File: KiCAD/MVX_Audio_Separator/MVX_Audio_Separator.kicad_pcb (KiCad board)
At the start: 2 copper layers, 30.9 x 26.9 mm, 4 parts, among them J1 3.5mm_vertical, P1 VGA_Female, P2 VGA_Male

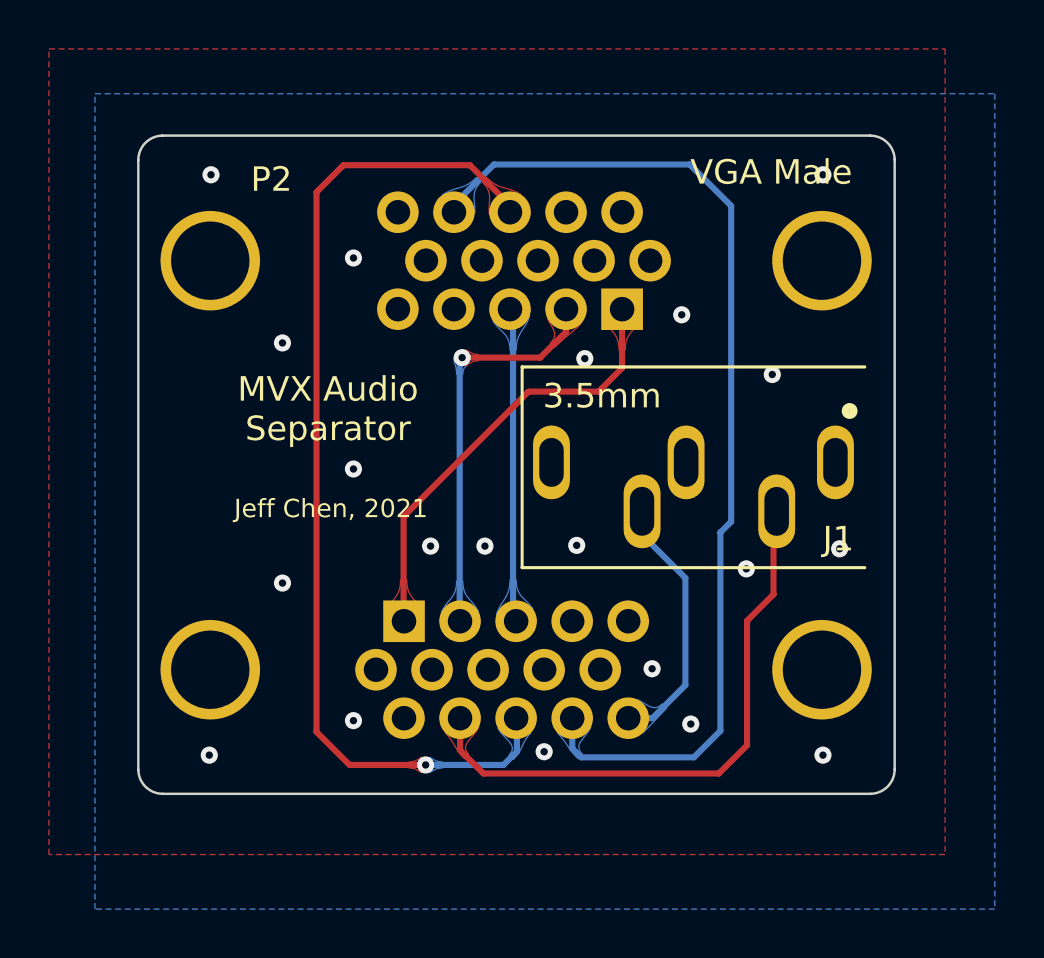
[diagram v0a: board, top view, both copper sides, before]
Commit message: Update PCB
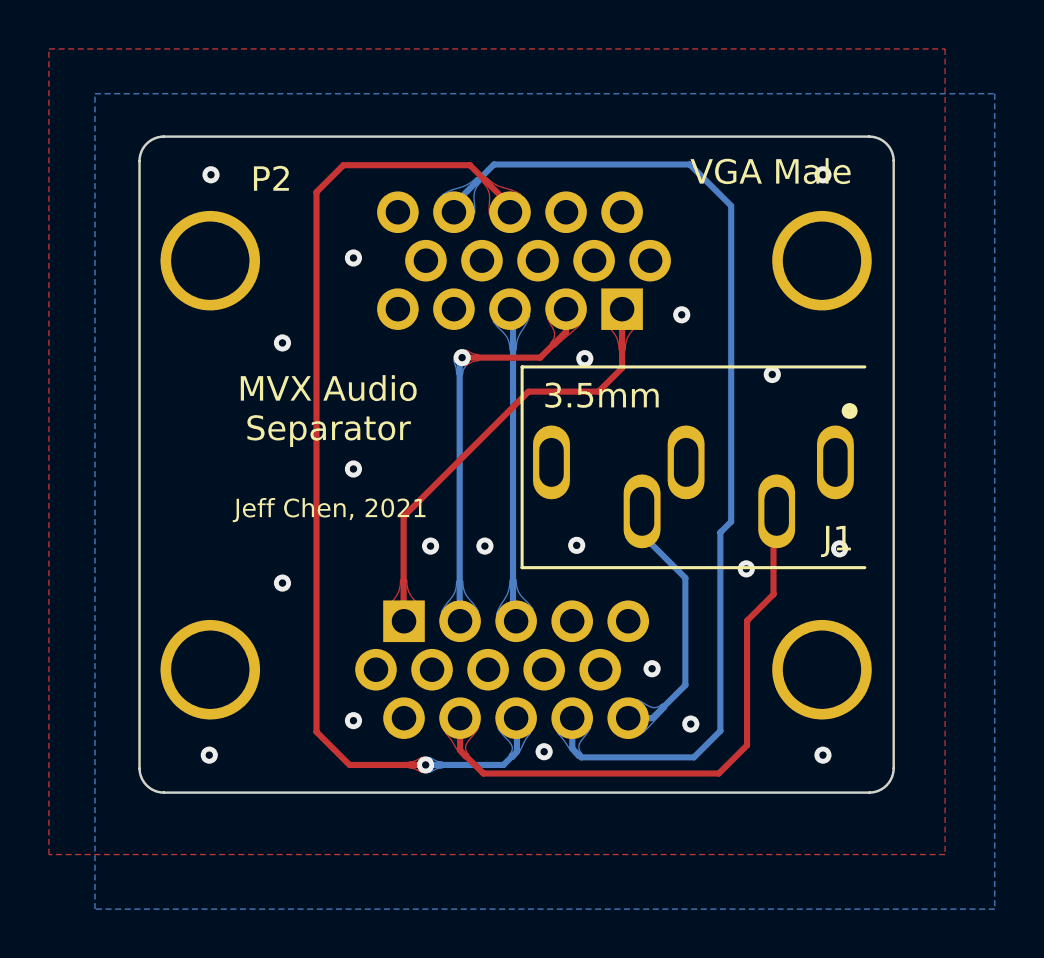
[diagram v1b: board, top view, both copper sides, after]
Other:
- board size 30.9 x 26.9 mm -> 30.8 x 26.8 mm
